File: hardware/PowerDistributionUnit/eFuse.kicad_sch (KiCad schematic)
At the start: 42 parts, among them Q1 CSD18511Q5A, Q2 2N7002, U12 AD5258, U13 TPS25983

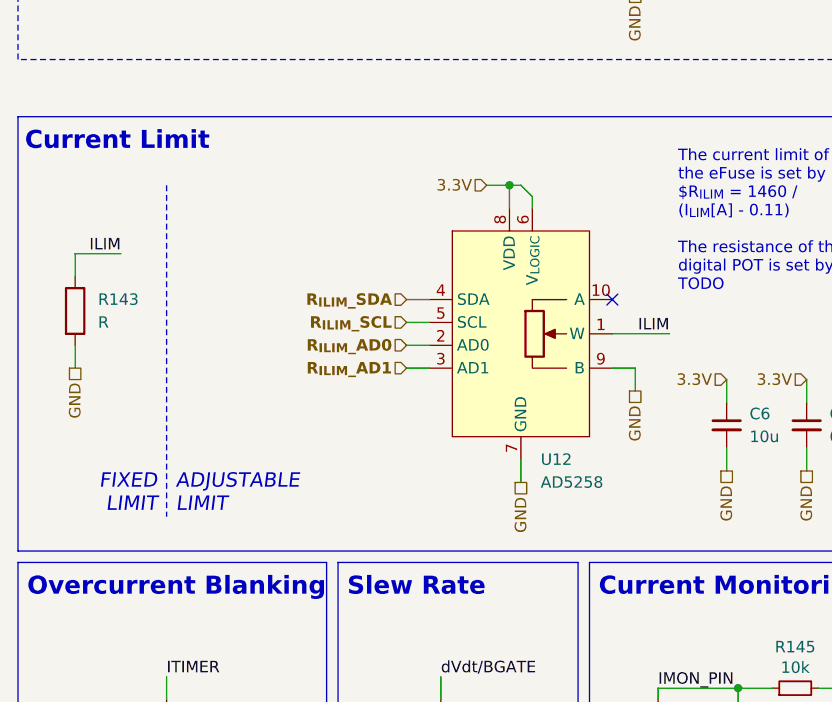
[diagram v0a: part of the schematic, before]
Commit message: redid multichannel
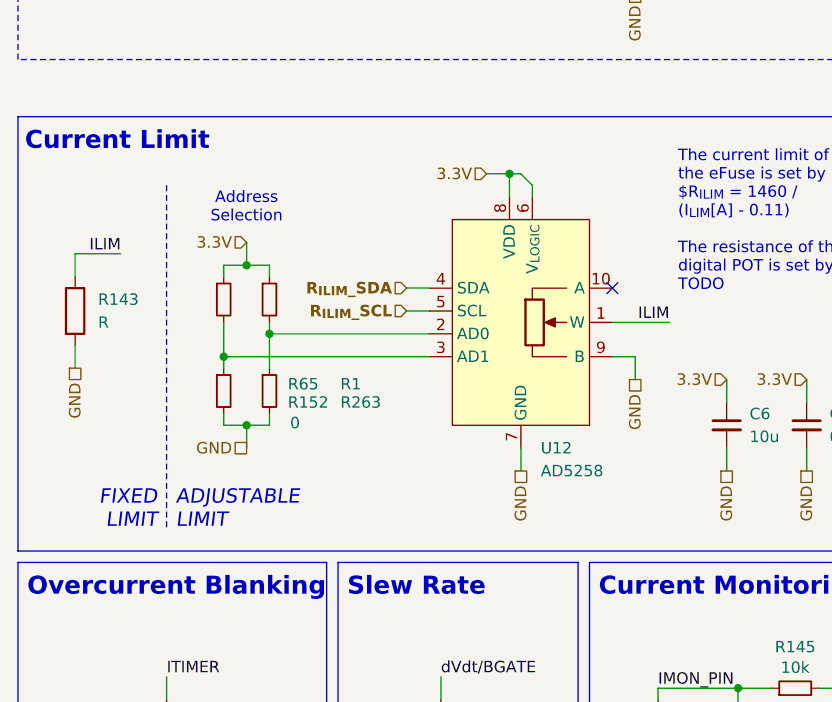
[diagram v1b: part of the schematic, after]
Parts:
- added R1, R152, R263, R65: 0, Resistor_SMD:R_0603_1608Metric, symbol Device:R_Small
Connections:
- net 3.3V: now also R1.1, R65.1
- net GND: now also R152.2, R263.2
- net R_{ILIM}_AD0: no longer names the net of U12.2 (AD0)
- net R_{ILIM}_AD0: now also R1.2, R263.1
- net R_{ILIM}_AD1: no longer names the net of U12.3 (AD1)
- net R_{ILIM}_AD1: now also R152.1, R65.2
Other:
- note added: "Address Selection"
- moved on the sheet: U12
